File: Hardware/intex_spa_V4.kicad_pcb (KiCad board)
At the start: 2 copper layers, 113 parts, among them U1 INA219BIDCNT

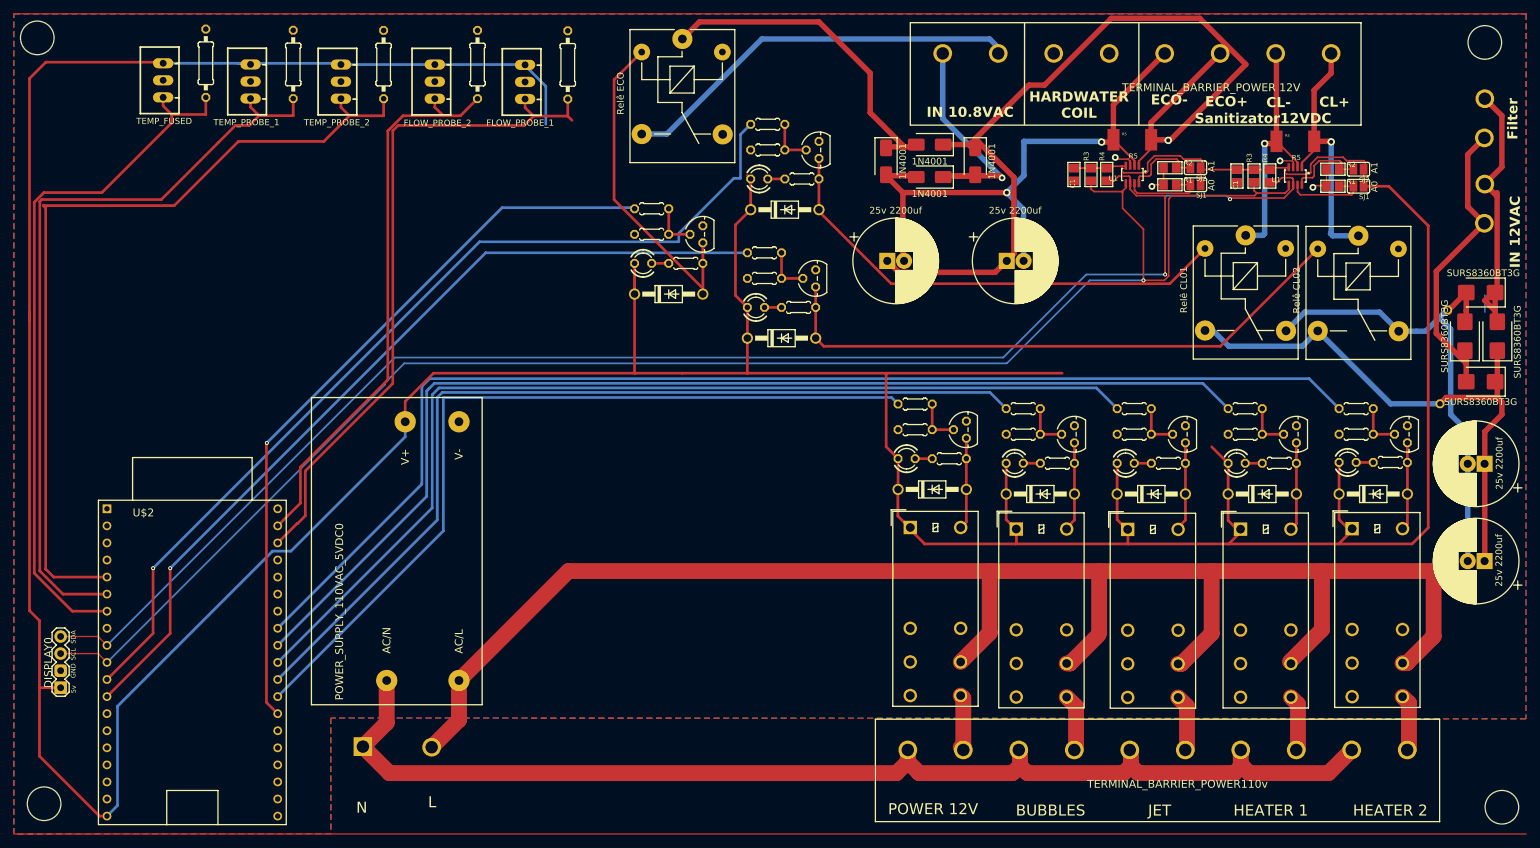
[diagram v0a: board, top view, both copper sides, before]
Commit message: Final HW  Hardware
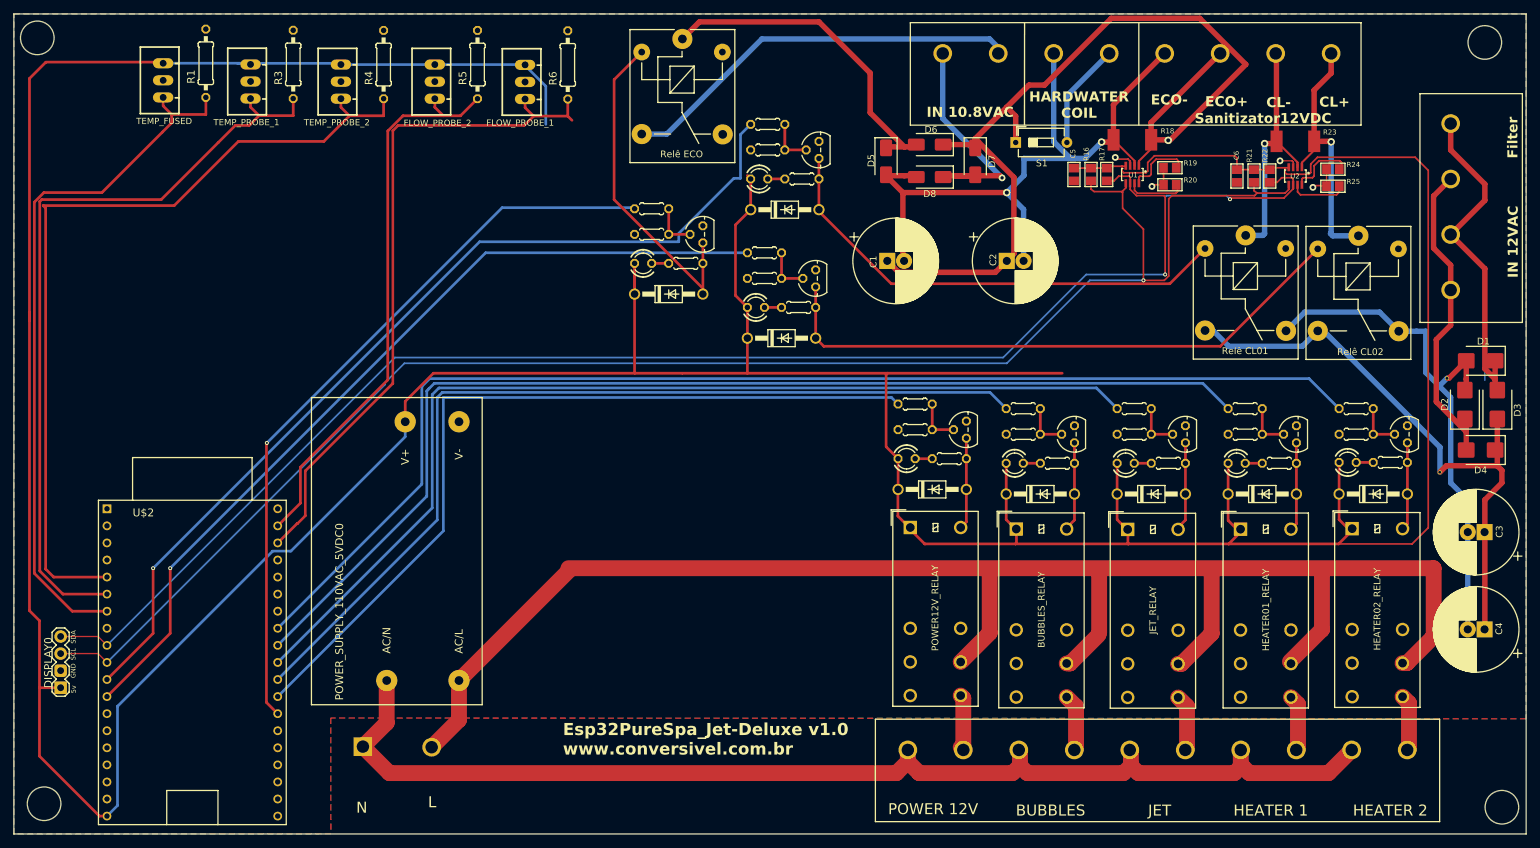
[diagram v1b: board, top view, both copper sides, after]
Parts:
- removed the ? at (239.7, 89.8)
- removed the ? at (240.8, 75.9)
- removed the ? at (246.4, 44.5)
- removed the ? at (246.3, 50.3)
- removed the ? at (246.3, 63.0)
- removed the ? at (246.4, 57.1)
- removed SJ1 (x2), SJ2 (x2): , Adafruit_INA219_CurPowerMonitor:SOLDERJUMPER_REFLOW_NOPASTE
- added ?: , , F.Cu at (239.7, 100.0)
- added ?: , , F.Cu at (240.8, 86.0)
- added S1: SW_DIP_SPSTx01_Slide_6.7x4.1mm_W7.62mm_P2.54mm_LowProfile, Button_Switch_THT:SW_DIP_SPSTx01_Slide_6.7x4.1mm_W7.62mm_P2.54mm_LowProfile, F.Cu at (176.6, 51.0)
- added TERMINAL_BARRIER_POWER 12V: 4PCV-04-006, intex_spa_V4:4PCV-04-006, F.Cu at (246.4, 36.1)
- C1, C2, C3, C4: renamed from 25v 2200uf
- D1, D2, D3, D4: renamed from SURS8360BT3G; value D_SMB -> SURS8360BT3G
- D5, D6, D7, D8: renamed from 1N4001; value D_SMA -> 1N4001
- moved C3 10.2 mm to (246.3, 108.9)
- moved C4 10.2 mm to (246.3, 123.4)
- moved D1 10.2 mm to (245.8, 83.4)
- moved D2 10.2 mm to (243.4, 89.9)
- moved D3 10.2 mm to (248.2, 89.9)
- moved D4 10.2 mm to (245.8, 96.7)
- renumbered C1 to C5, C1 to C6, HEATER_2_RELAY_DIODE0 to D10, HEATER_2_RELAY_DIODE0 to D11, HEATER_2_RELAY_DIODE0 to D12, HEATER_1_RELAY_DIODE0 to D13, JET_RELAY_DIODE0 to D14, PUMP_RELAY_DIODE0 to D15, HEATER_2_RELAY_DIODE0 to D8, HEATER_2_RELAY_DIODE0 to D9, PUMP0 to LED1, PUMP0 to LED_BUBBLES_RELAY, HEATER_1 to LED_HEATER1_RELAY, HEATER_2 to LED_HEATER2_RELAY, PUMP0 to LED_RELAY_CL1, PUMP0 to LED_RELAY_CL2, R_FLOW_1 to R1, R_PUMP_RELAY0 to R10, R_PUMP_RELAY1 to R11, R_LED_JET2 to R12, R_PUMP_RELAY0 to R13, R_PUMP_RELAY1 to R14, R_LED_JET2 to R15, R3 to R16, R4 to R17, R5 to R18, R2 to R19, R1 to R20, R3 to R21, R4 to R22, R5 to R23, R2 to R24, R_PUMP_RELAY0 to R24, R1 to R25, R_PUMP_RELAY1 to R25, R_LED_JET2 to R26, R_PUMP_RELAY0 to R27, R_PUMP_RELAY1 to R28, R_LED_JET2 to R29, R_FLOW_1 to R3, R_PUMP_RELAY2 to R30, R_PUMP_RELAY3 to R31, R_LED_JET1 to R32, R_PUMP_RELAY4 to R33, R_PUMP_RELAY6 to R34, R_LED_JET0 to R35, R_PUMP_RELAY5 to R36, R_PUMP_RELAY7 to R37, R_LED_PUMP0 to R38, R_FLOW_1 to R4, R_FLOW_2 to R5, R_FLOW_1 to R6, R_PUMP_RELAY0 to R7, R_PUMP_RELAY1 to R8, R_LED_JET2 to R9, T_PUMP_RELAY0 to T_BUBBLES_RELAY, T_PUMP_RELAY3 to T_HEATER2_RELAY, T_PUMP_RELAY0 to T_RELAY_CL1, T_PUMP_RELAY0 to T_RELAY_CL2, T_PUMP_RELAY0 to T_RELAY_ECO, T_PUMP_RELAY2 to T__HEATER1_RELAY, U1 to U2
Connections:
- BUBBLES_RELAY pad A2: (no net) -> A_BUBBLES
- LED1 pad K: N$14 -> N$15
- R7 pad 1: N$13 -> N$16
- R8 pad 1: N$13 -> N$16
- R9 pad 1: N$14 -> N$15
- TERMINAL_BARRIER_POWER 12V pad I3: (no net) -> 12VDC-
- TERMINAL_BARRIER_POWER 12V pad I4: (no net) -> 12VDC+
- T_RELAY_ECO pad 2: N$13 -> N$16
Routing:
- net 12VDC+: track 219.5 -> 248.5 mm
- net 12VDC-: track 161.6 -> 183.4 mm
- net 12VAC+: track 40.5 -> 49.1 mm
- net N$16: track 0.00 -> 6.98 mm
- net N$13: track 14.0 -> 6.99 mm
- net I1_ELT2: track 12.8 -> 8.48 mm
- net I1_ELT1: track 12.8 -> 8.83 mm
- net +5V: track 714.0 -> 710.5 mm
- net N$15: track 0.00 -> 2.54 mm
- net N$14: track 5.08 -> 2.54 mm
- net I2_ELT2: track 12.3 -> 10.2 mm
- net I2_ELT1: track 12.3 -> 10.2 mm
- net 12VAC_N: track 45.1 -> 47.1 mm
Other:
- board outline added: 225 x 122 mm
- board text added: "Esp32PureSpa_Jet-Deluxe v1.0 www.conversivel.com.br"
- board text added: "R18"
- board text added: "R23"
- board text removed: "A0"
- board text removed: "A1"
- board text removed: "R5"
